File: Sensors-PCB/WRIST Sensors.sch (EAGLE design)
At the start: 13 parts, among them U1 VL6180X, U10 VL6180X, U2 VL6180X, U3 VL6180X, U4 VL6180X, U5 VL6180X, U6 VL6180X, U7 VL6180X, U8 VL6180X, U9 VL6180X

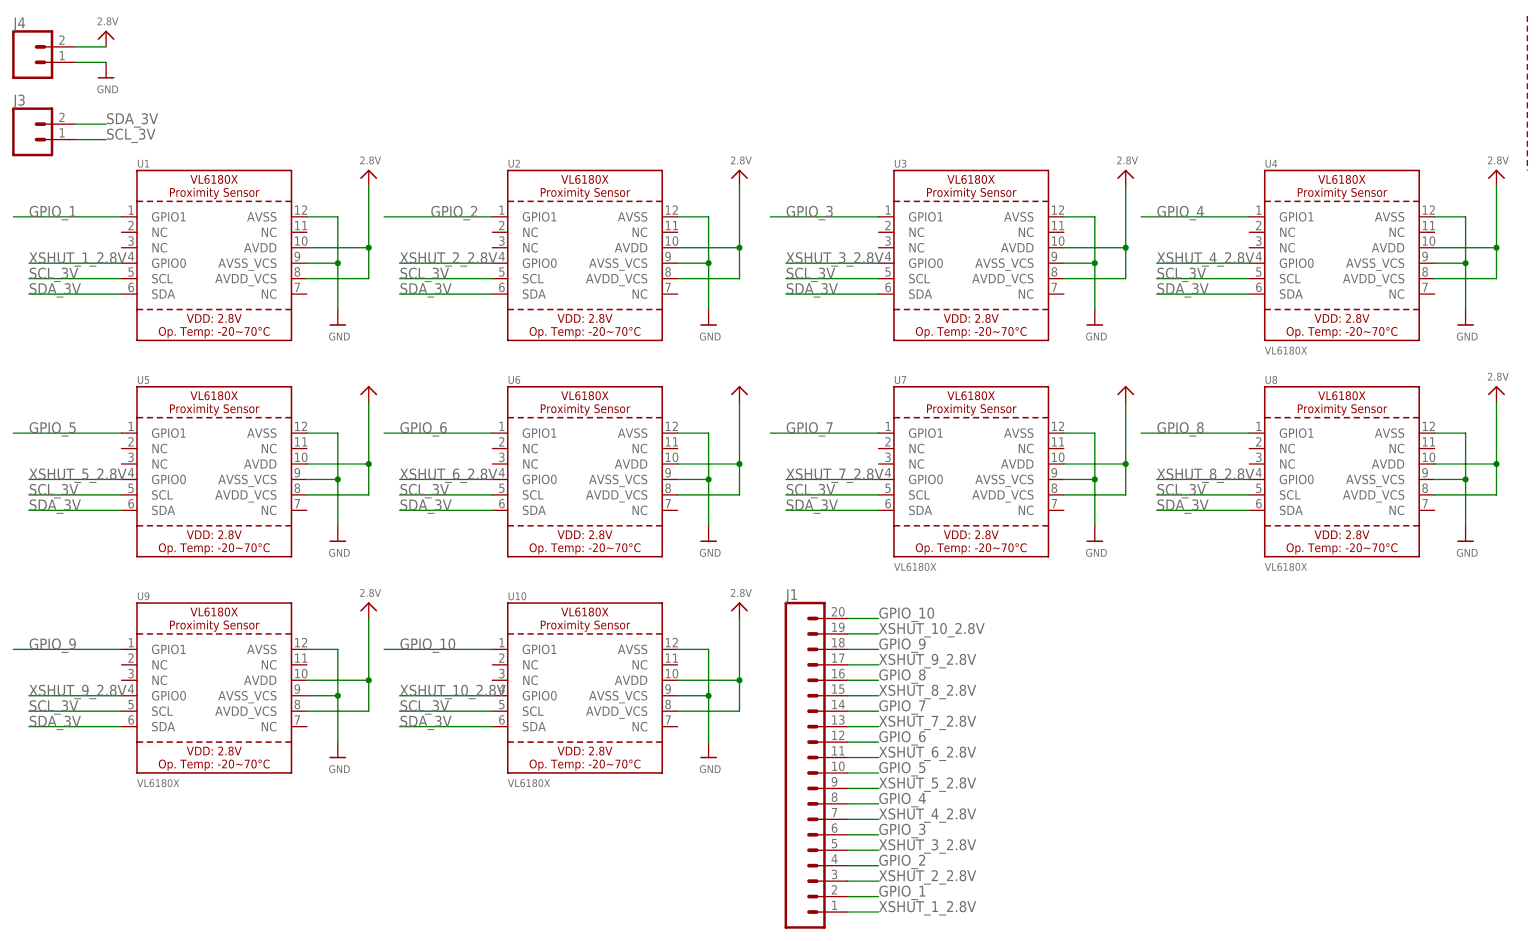
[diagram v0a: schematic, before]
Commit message: progress
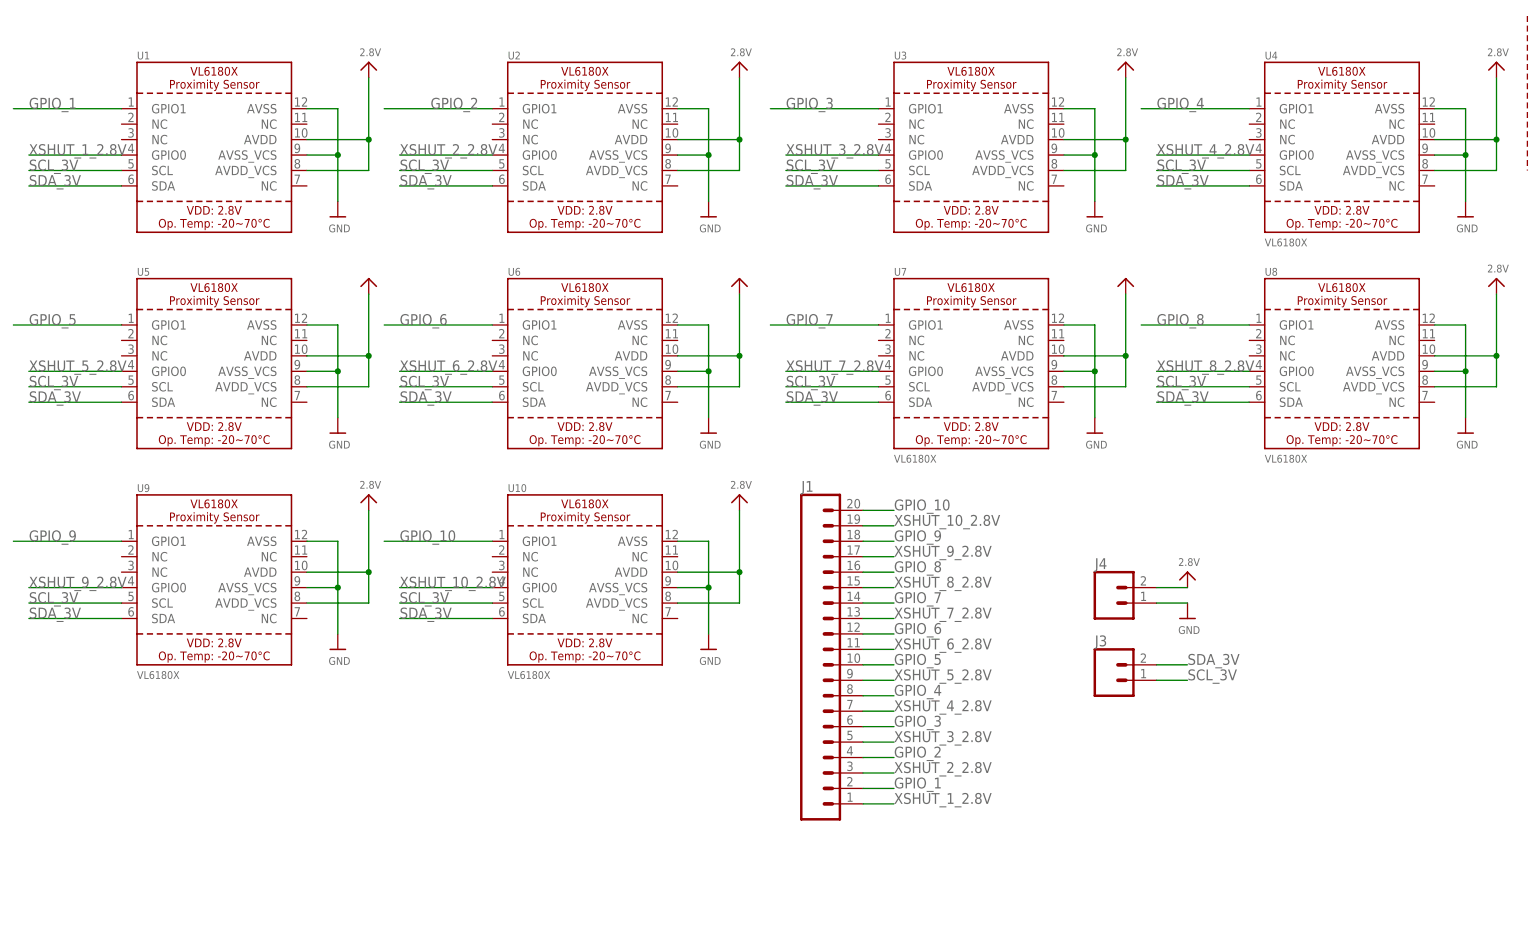
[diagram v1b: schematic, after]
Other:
- moved on the sheet: J1, J3, J4, U1, U10, U2, U3, U4, U5, U6, U7, U8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
